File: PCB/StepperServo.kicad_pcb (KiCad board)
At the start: 2 copper layers, 56 x 56 mm, 69 parts, among them P1 Conn_01x06, P2 Conn_01x04, P4 Conn_01x08, P5 Conn_01x02, U1 AOZ1282CI, U2 A4950E, U4 A4950E, U5 TLE5012B, U7 STM32F103CBTx, U8 LD1117S33CTR, U9 PCA82C251, Y1 Crystal, p7 Conn_01x08

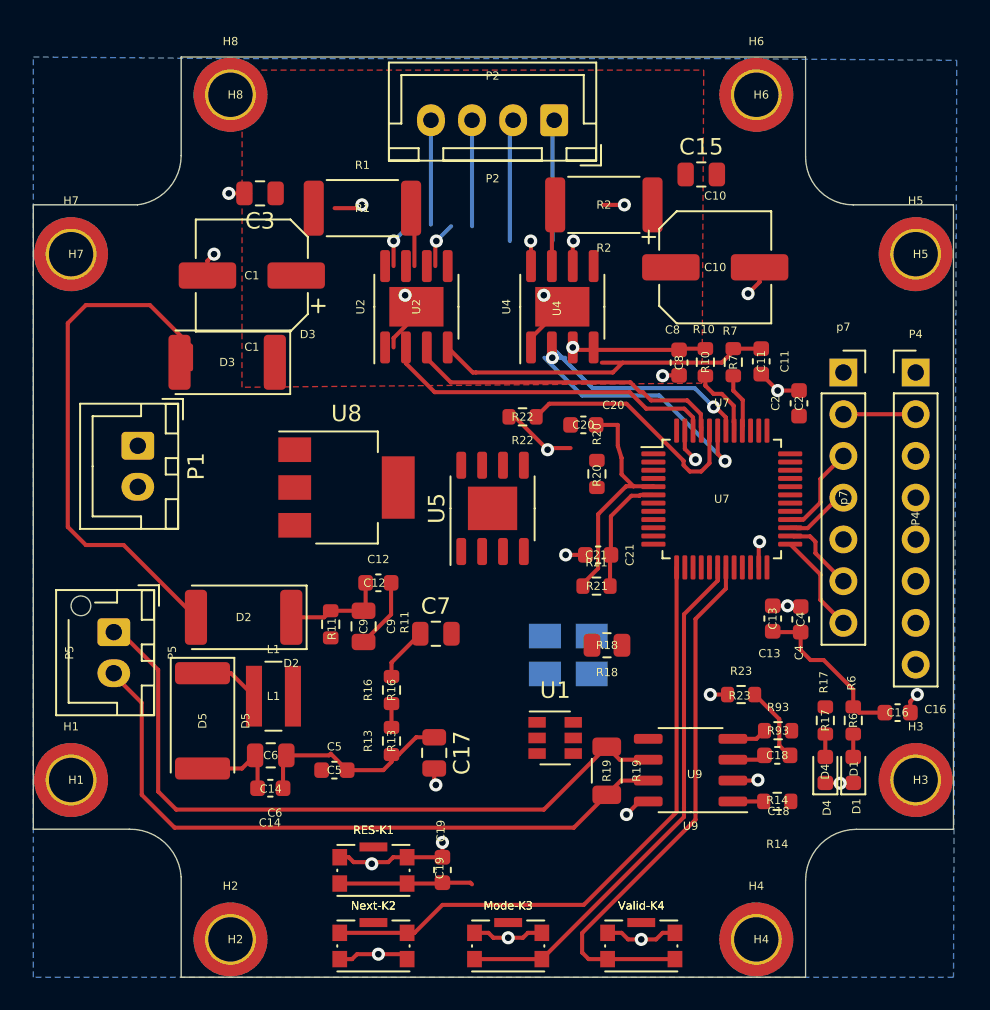
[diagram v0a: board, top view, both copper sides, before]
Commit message: Kicad 6
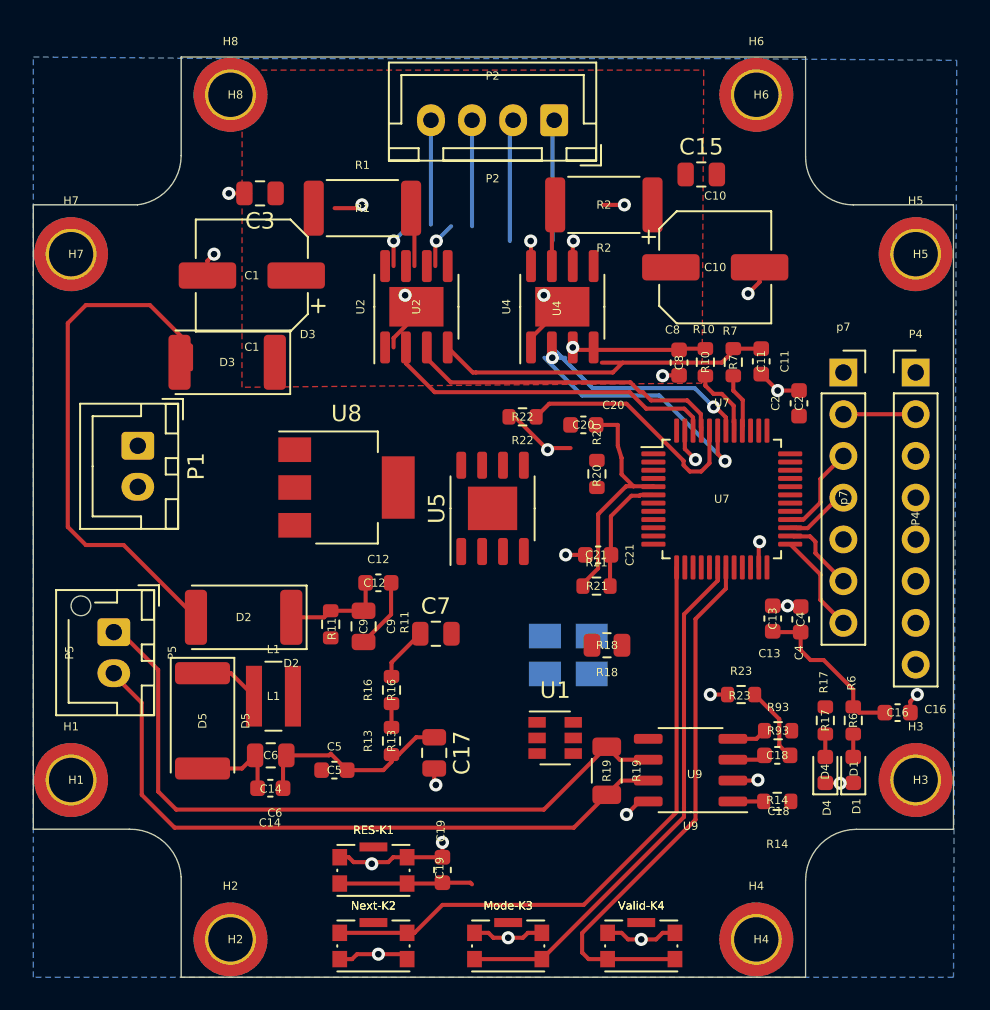
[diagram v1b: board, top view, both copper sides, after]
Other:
- net class Default removed
